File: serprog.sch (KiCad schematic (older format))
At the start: 42 parts, among them J1 USB_B_Micro, SW1 SW_Push_SPDT, U1 TXS0108EPW, U2 XC6206PxxxMR1v8, U3 XC6206PxxxMR3v3, U4 AT25xxx, U5 STM32F102R8Tx, Y1 8M

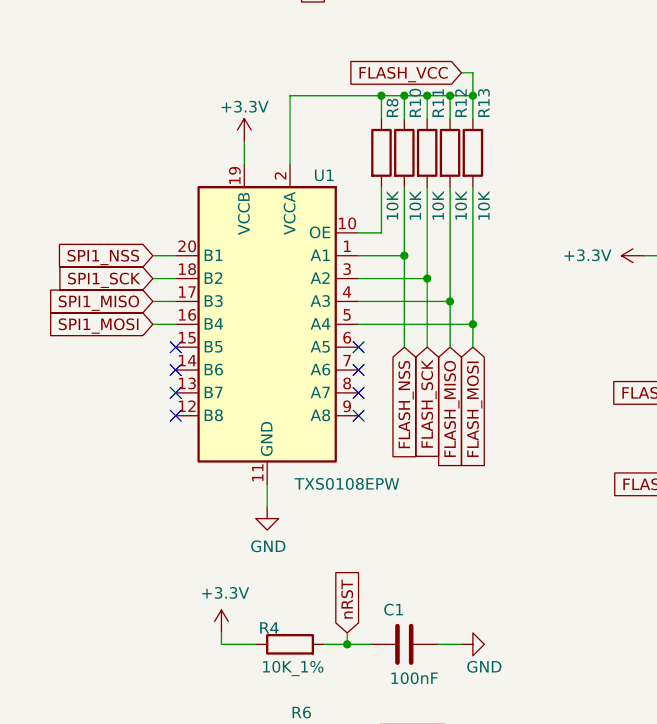
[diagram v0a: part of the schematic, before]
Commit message: v0.2
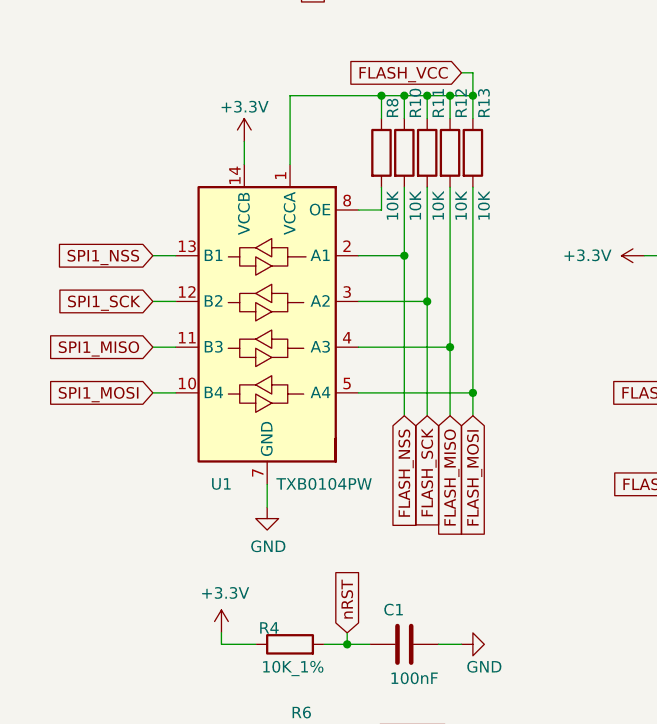
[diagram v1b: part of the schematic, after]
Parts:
- removed U1: TXS0108EPW, Package_SO:TSSOP-20_4.4x6.5mm_P0.65mm, symbol Logic_LevelTranslator:TXS0108EPW
- added U1: TXB0104PW, Package_SO:TSSOP-14_4.4x5mm_P0.65mm, symbol Logic_LevelTranslator:TXB0104PW
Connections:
- net +3V3: now also U1.14 (VCCB)
- net FLASH_MISO: now also U1.4 (A3)
- net FLASH_MOSI: now also U1.5 (A4)
- net FLASH_NSS: now also U1.2 (A1)
- net FLASH_SCK: now also U1.3 (A2)
- net FLASH_VCC: now also U1.1 (VCCA)
- net GND: now also U1.7 (GND)
- net SPI1_MISO: now also U1.11 (B3)
- net SPI1_MOSI: now also U1.10 (B4)
- net SPI1_NSS: now also U1.13 (B1)
- net SPI1_SCK: now also U1.12 (B2)
- net at R8.2: now also U1.8 (OE)
- no-connect marks 47 -> 39
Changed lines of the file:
@@
 	3600 5250 3700 5250
 $Comp
-L power:+3.3V #PWR026
+L power:+3.3V #PWR025
 U 1 1 60A418C5
 P 8000 1300
-F 0 "#PWR026" H 8000 1150 50  0001 C CNN
+F 0 "#PWR025" H 8000 1150 50  0001 C CNN
 F 1 "+3.3V" H 8015 1473 50  0000 C CNN
 F 2 "" H 8000 1300 50  0001 C CNN
@@
 	8100 1400 8200 1400
 $Comp
-L power:GND #PWR027
+L power:GND #PWR026
 U 1 1 60A4D3BD
 P 8000 5300
-F 0 "#PWR027" H 8000 5050 50  0001 C CNN
+F 0 "#PWR026" H 8000 5050 50  0001 C CNN
 F 1 "GND" H 8005 5127 50  0000 C CNN
 F 2 "" H 8000 5300 50  0001 C CNN
@@
 	6100 6500 6400 6500
 $Comp
-L power:+3.3V #PWR024
+L power:+3.3V #PWR023
 U 1 1 60A95BE4
 P 6400 5950
-F 0 "#PWR024" H 6400 5800 50  0001 C CNN
+F 0 "#PWR023" H 6400 5800 50  0001 C CNN
 F 1 "+3.3V" H 6400 6100 50  0000 C CNN
 F 2 "" H 6400 5950 50  0001 C CNN
@@
 $EndComp
 $Comp
-L power:GND #PWR025
+L power:GND #PWR024
 U 1 1 60A96AE9
 P 6400 6500
-F 0 "#PWR025" H 6400 6250 50  0001 C CNN
+F 0 "#PWR024" H 6400 6250 50  0001 C CNN
 F 1 "GND" H 6405 6327 50  0000 C CNN
 F 2 "" H 6400 6500 50  0001 C CNN
@@
 Text GLabel 2750 3550 0    50   Input ~ 0
 SPI1_NSS
-Text GLabel 2750 3650 0    50   Input ~ 0
+Text GLabel 2750 3750 0    50   Input ~ 0
 SPI1_SCK
-Text GLabel 2750 3750 0    50   Input ~ 0
+Text GLabel 2750 3950 0    50   Input ~ 0
 SPI1_MISO
-Text GLabel 2750 3850 0    50   Input ~ 0
+Text GLabel 2750 4150 0    50   Input ~ 0
 SPI1_MOSI
 $Comp
@@
 	5300 4350 5300 4150
 $Comp
-L power:+3.3V #PWR021
+L power:+3.3V #PWR020
 U 1 1 60A68DEC
 P 6000 3700
-F 0 "#PWR021" H 6000 3550 50  0001 C CNN
+F 0 "#PWR020" H 6000 3550 50  0001 C CNN
 F 1 "+3.3V" V 6000 3950 50  0000 C CNN
 F 2 "" H 6000 3700 50  0001 C CNN
@@
 $EndComp
 $Comp
-L power:+1V8 #PWR022
+L power:+1V8 #PWR021
 U 1 1 60A6EB3A
 P 6000 3900
-F 0 "#PWR022" H 6000 3750 50  0001 C CNN
+F 0 "#PWR021" H 6000 3750 50  0001 C CNN
 F 1 "+1V8" V 6000 4150 50  0000 C CNN
 F 2 "" H 6000 3900 50  0001 C CNN
@@
 	5300 3550 5500 3550
 $Comp
-L power:GND #PWR023
+L power:GND #PWR022
 U 1 1 60AA905C
 P 6100 3550
-F 0 "#PWR023" H 6100 3300 50  0001 C CNN
+F 0 "#PWR022" H 6100 3300 50  0001 C CNN
 F 1 "GND" V 6100 3350 50  0000 C CNN
 F 2 "" H 6100 3550 50  0001 C CNN
@@
 Wire Wire Line
 	5500 3550 5700 3550
-$Comp
-L Logic_LevelTranslator:TXS0108EPW U1
-U 1 1 60AF84A4
-P 3250 3850
-F 0 "U1" H 3000 4500 50  0000 C CNN
-F 1 "TXS0108EPW" H 2900 3150 50  0000 C CNN
-F 2 "Package_SO:TSSOP-20_4.4x6.5mm_P0.65mm" H 3250 3100 50  0001 C CNN
-F 3 "www.ti.com/lit/ds/symlink/txs0108e.pdf" H 3250 3750 50  0001 C CNN
-	1    3250 3850
-	-1   0    0    -1
-$EndComp
 Wire Wire Line
 	5250 4150 5300 4150
@@
 Wire Wire Line
 	3250 4550 3250 4650
-Text GLabel 3850 3950 3    50   Input ~ 0
+Text GLabel 3850 4250 3    50   Input ~ 0
 FLASH_NSS
-Text GLabel 3950 3950 3    50   Input ~ 0
+Text GLabel 3950 4250 3    50   Input ~ 0
 FLASH_SCK
-Text GLabel 4150 3950 3    50   Input ~ 0
+Text GLabel 4150 4250 3    50   Input ~ 0
 FLASH_MOSI
-Text GLabel 4050 3950 3    50   Input ~ 0
+Text GLabel 4050 4250 3    50   Input ~ 0
 FLASH_MISO
 Text GLabel 5250 4550 0    50   Input ~ 0
@@
 Text GLabel 6150 4550 2    50   Input ~ 0
 FLASH_MISO
-NoConn ~ 2850 3950
-NoConn ~ 2850 4050
-NoConn ~ 2850 4150
-NoConn ~ 2850 4250
-NoConn ~ 3650 3950
-NoConn ~ 3650 4050
-NoConn ~ 3650 4150
-NoConn ~ 3650 4250
 Wire Wire Line
 	3650 3550 3850 3550
-Wire Wire Line
-	3650 3650 3950 3650
-Wire Wire Line
-	3650 3750 4050 3750
-Wire Wire Line
-	3650 3850 4150 3850
 $Comp
 L Device:R R10
@@
 $EndComp
 Wire Wire Line
-	3750 3250 3750 3450
-Wire Wire Line
-	3750 3450 3650 3450
-Wire Wire Line
 	3850 3250 3850 3550
-Connection ~ 3850 3550
-Wire Wire Line
-	3850 3550 3850 3950
-Wire Wire Line
-	3950 3250 3950 3650
-Connection ~ 3950 3650
-Wire Wire Line
-	3950 3650 3950 3950
-Wire Wire Line
-	4050 3250 4050 3750
-Connection ~ 4050 3750
-Wire Wire Line
-	4050 3750 4050 3950
-Wire Wire Line
-	4150 3250 4150 3850
-Connection ~ 4150 3850
-Wire Wire Line
-	4150 3850 4150 3950
 Wire Wire Line
 	3750 2950 3750 2850
@@
 	2750 3550 2850 3550
 Wire Wire Line
-	2850 3650 2750 3650
-Wire Wire Line
-	2750 3750 2850 3750
-Wire Wire Line
-	2850 3850 2750 3850
+	2850 3750 2750 3750
+Wire Wire Line
+	2750 3950 2850 3950
+Wire Wire Line
+	2850 4150 2750 4150
 $Comp
 L power:+3.3V #PWR03
@@
 $EndComp
 $Comp
-L power:GND #PWR020
+L power:GND #PWR019
 U 1 1 60CFA445
 P 5900 2850
-F 0 "#PWR020" H 5900 2600 50  0001 C CNN
+F 0 "#PWR019" H 5900 2600 50  0001 C CNN
 F 1 "GND" V 5905 2722 50  0000 R CNN
 F 2 "" H 5900 2850 50  0001 C CNN
@@
 $EndComp
 $Comp
-L power:GND #PWR019
+L power:GND #PWR018
 U 1 1 60D095DF
 P 5900 2450
-F 0 "#PWR019" H 5900 2200 50  0001 C CNN
+F 0 "#PWR018" H 5900 2200 50  0001 C CNN
 F 1 "GND" V 5905 2322 50  0000 R CNN
 F 2 "" H 5900 2450 50  0001 C CNN
@@
 	0    -1   -1   0
 $EndComp
+$Comp
+L Logic_LevelTranslator:TXB0104PW U1
+U 1 1 60AC3318
+P 3250 3850
+F 0 "U1" H 3450 3150 50  0000 C CNN
+F 1 "TXB0104PW" H 3000 3150 50  0000 C CNN
+F 2 "Package_SO:TSSOP-14_4.4x5mm_P0.65mm" H 3250 3100 50  0001 C CNN
+F 3 "http://www.ti.com/lit/ds/symlink/txb0104.pdf" H 3360 3945 50  0001 C CNN
+	1    3250 3850
+	-1   0    0    -1
+$EndComp
+Wire Wire Line
+	3850 3550 3850 4250
+Connection ~ 3850 3550
+Wire Wire Line
+	3750 3250 3750 3350
+Wire Wire Line
+	3750 3350 3650 3350
+Wire Wire Line
+	3950 3250 3950 3750
+Wire Wire Line
+	3650 3750 3950 3750
+Connection ~ 3950 3750
+Wire Wire Line
+	3950 3750 3950 4250
+Wire Wire Line
+	3650 3950 4050 3950
+Wire Wire Line
+	4050 3250 4050 3950
+Connection ~ 4050 3950
+Wire Wire Line
+	4050 3950 4050 4250
+Wire Wire Line
+	3650 4150 4150 4150
+Wire Wire Line
+	4150 3250 4150 4150
+Connection ~ 4150 4150
+Wire Wire Line
+	4150 4150 4150 4250
 $EndSCHEMATC
